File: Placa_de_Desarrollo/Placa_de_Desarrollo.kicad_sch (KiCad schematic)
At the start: 44 parts, among them J1 USB_A, J10 Conn_01x04, J11 Conn_01x03, J12 Conn_01x04, J13 Conn_01x04, J14 Conn_01x04, J15 Conn_01x04, J16 Conn_01x04, J17 Conn_01x01, J18 Conn_01x01, J2 LEFT, J3 RIGHT, J4 Conn_01x01, J5 Conn_01x04, J6 Conn_01x04, J7 Conn_01x04, J8 Conn_01x03, J9 Conn_01x04, Q1 BC547, SW1 RESET, SW2 PULL DOWN, SW3 PULL UP, U2 RP2350

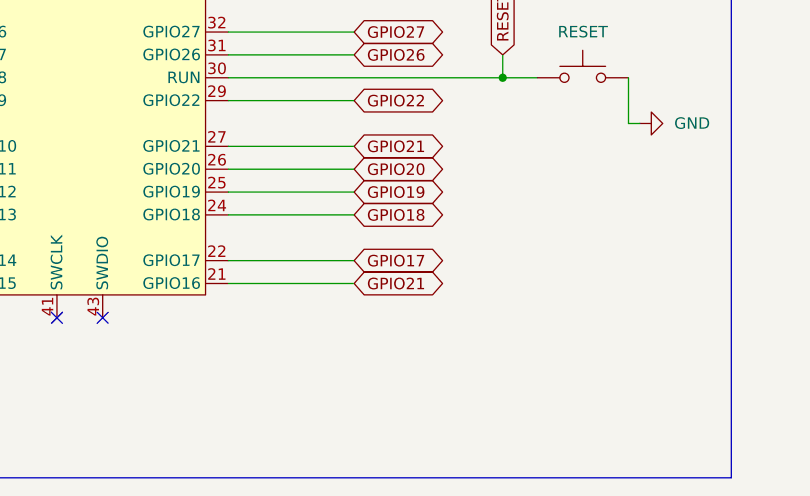
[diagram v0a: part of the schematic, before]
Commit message: Resguardo para actualizar KiCAD a version 10
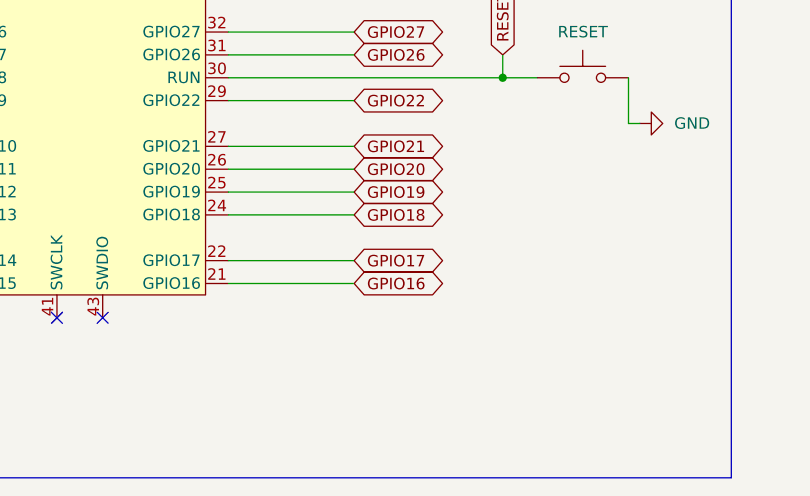
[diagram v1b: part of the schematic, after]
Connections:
- net GPIO16: now also U2.21 (GPIO16)
- net GPIO21: no longer U2.21 (GPIO16)
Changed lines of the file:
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@@
 		)
 	)
-	(global_label "GPIO21"
+	(global_label "GPIO16"
 		(shape bidirectional)
 		(at 88.9 176.53 0)
